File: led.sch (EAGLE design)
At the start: 47 parts, among them U1 TPS92513, U2 TPS92513

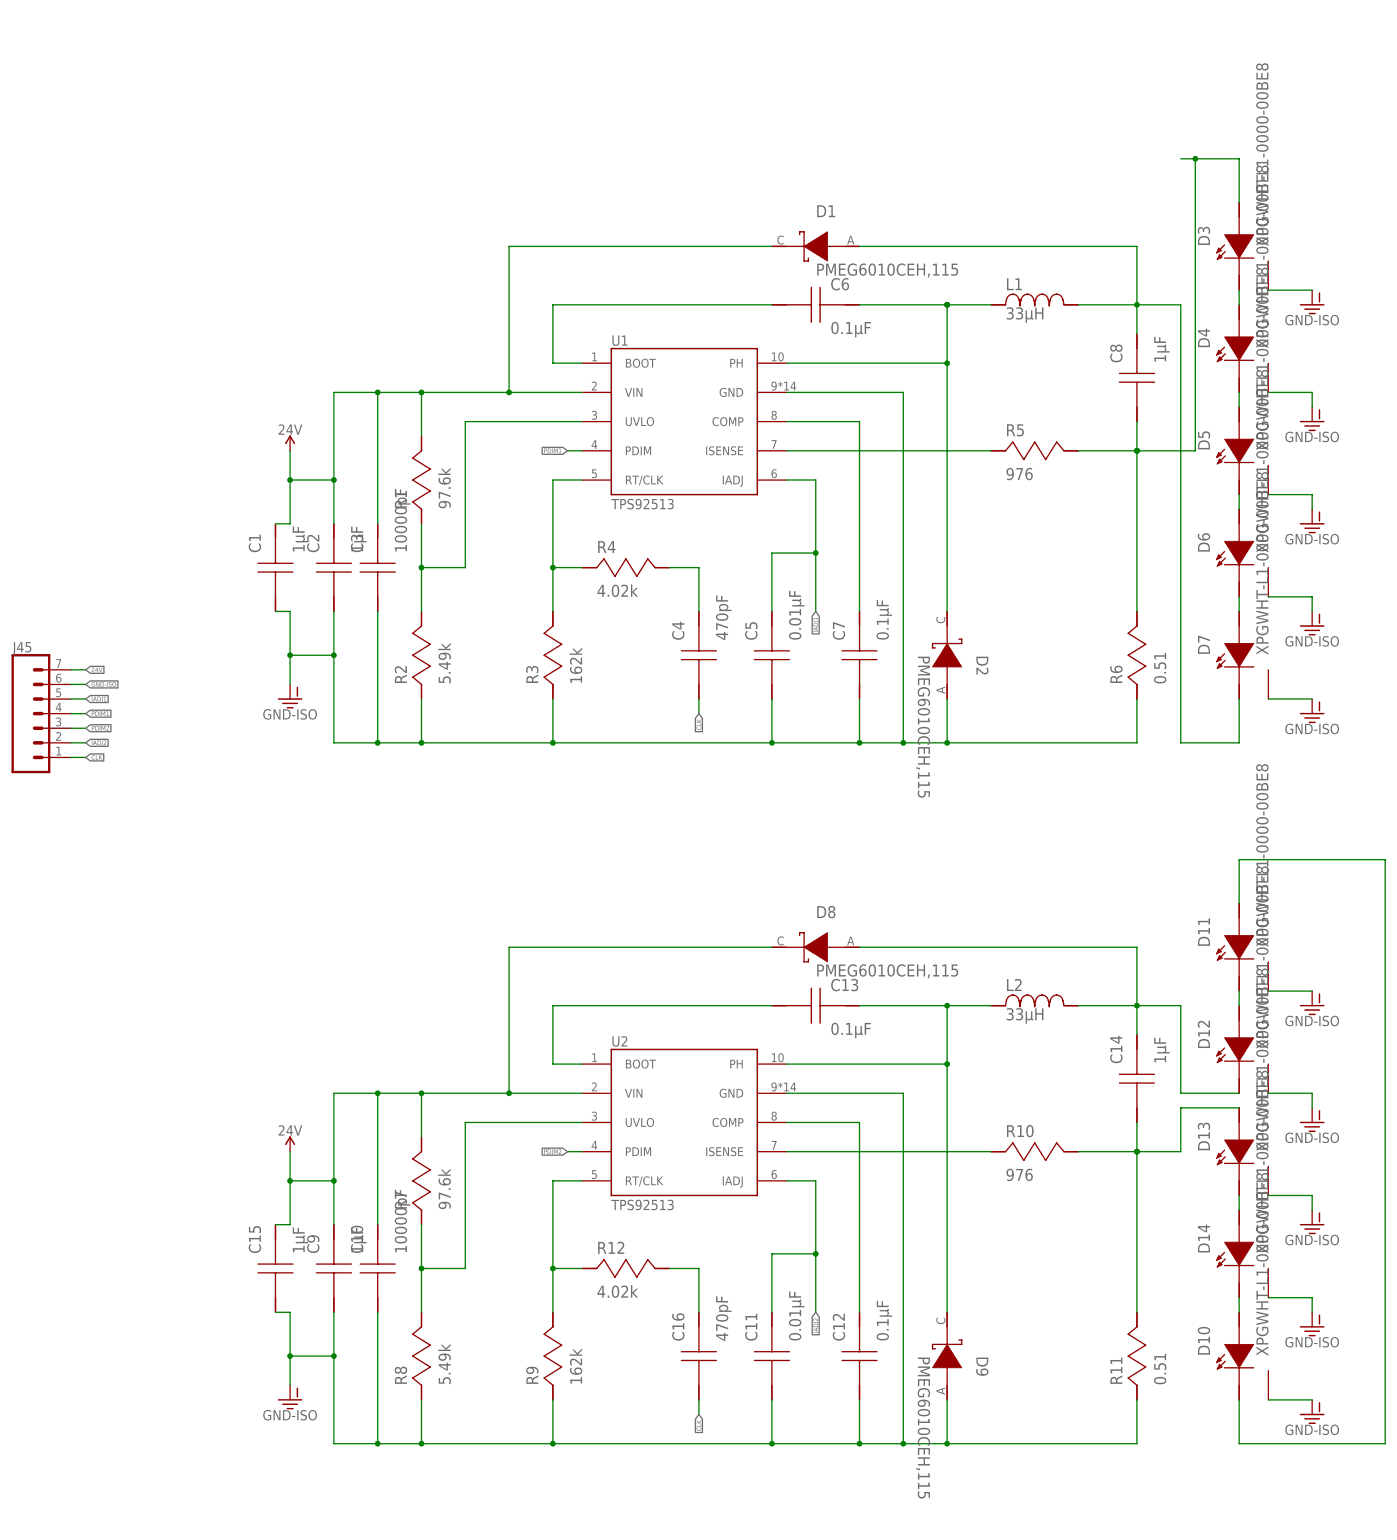
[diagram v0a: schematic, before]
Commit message: save
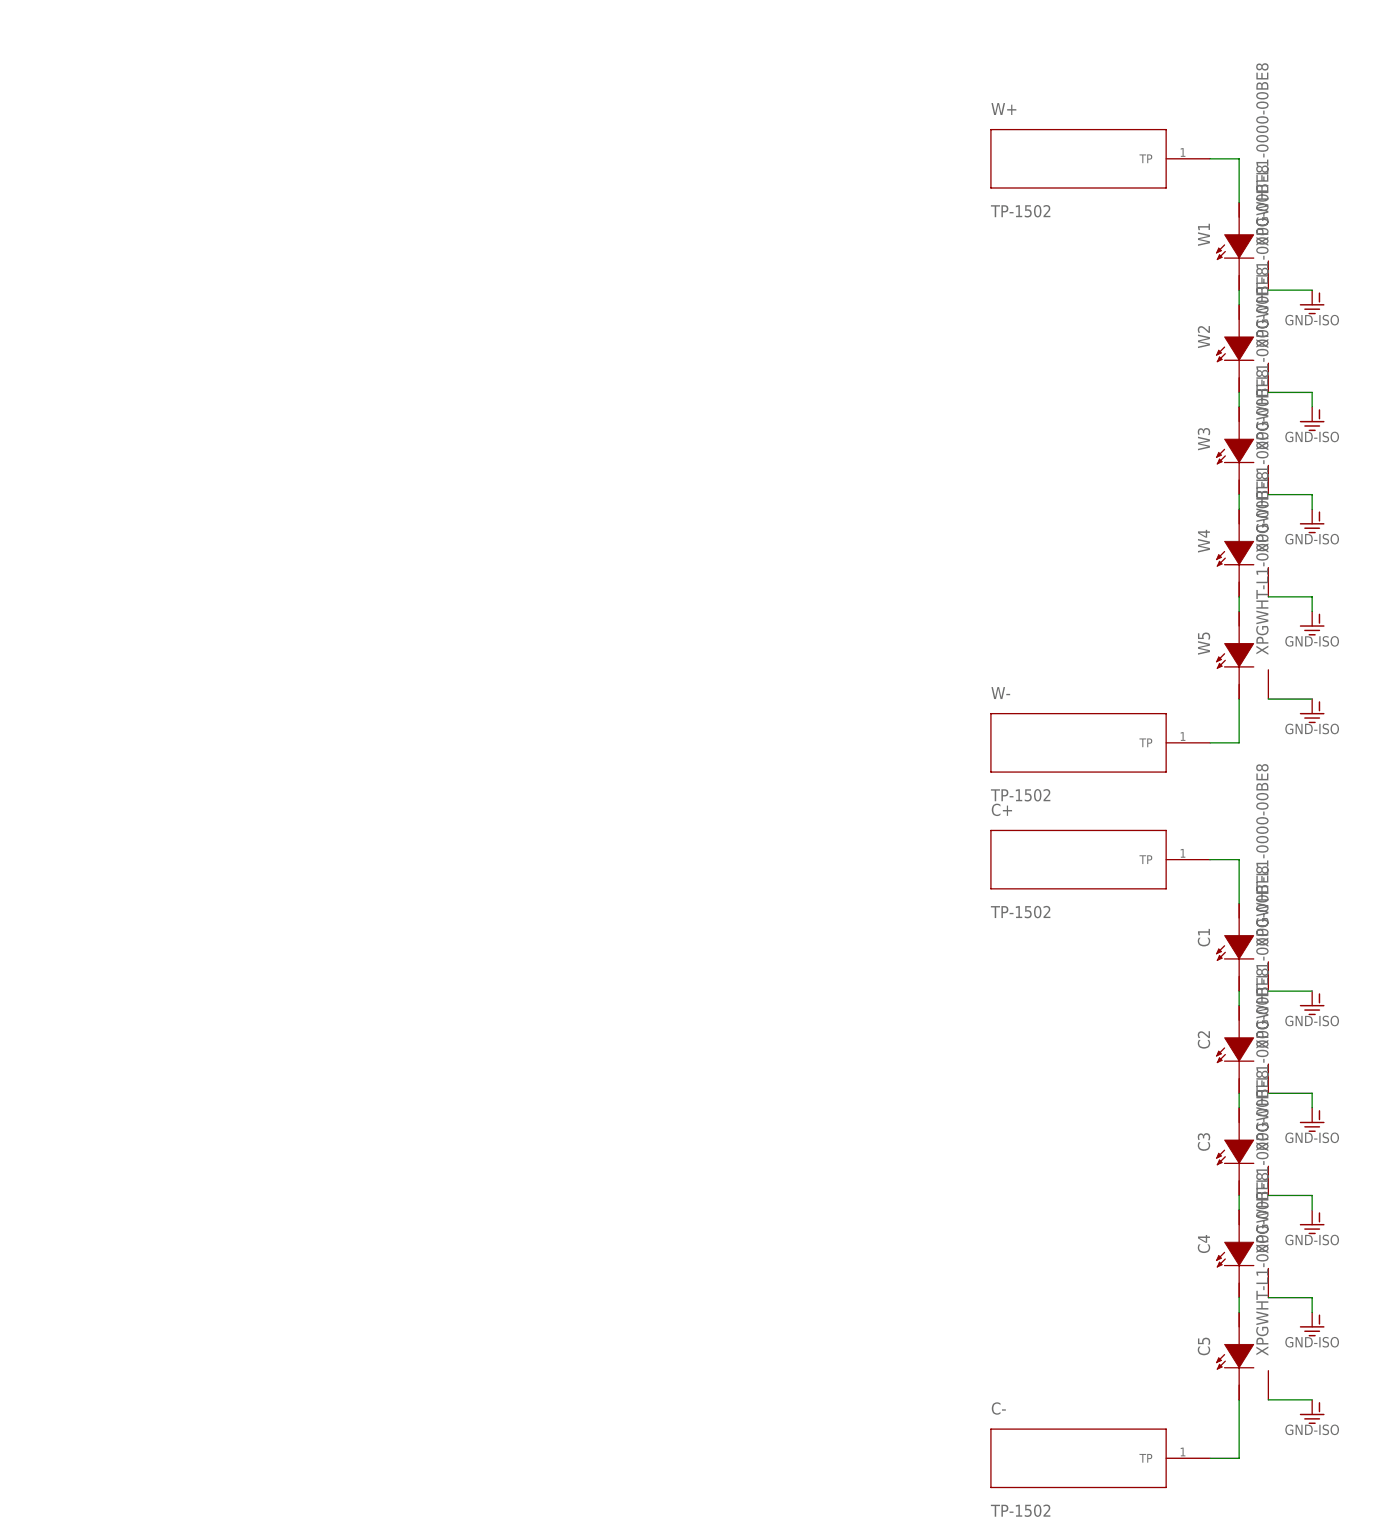
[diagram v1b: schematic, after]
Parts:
- removed C10: 10000pF, derek:GCM155R71H103KA55D
- removed C11: 0.01μF, derek:CC0805KRX7R9BB103
- removed C12, C7: 0.1µF, derek:CC0805KRX7R8BB104
- removed C13, C6: 0.1µF, derek:GRM188R71E104KA01D
- removed C14, C8: 1µF, derek:GMK212B7105KG-T
- removed C15, C9: 1µF, derek:GRM31MR71H105KA88L
- removed C16: 470pF, derek:C0603X471K5RACTU
- removed D1, D2, D8, D9: PMEG6010CEH,115, derek:PMEG6010CEH,115
- removed D10, D11, D12, D13, D14: XPGWHT-L1-0000-00BE8, derek:XPGWHT-L1-0000-00BE8
- removed J45: (no value), derek:CONN_07NO_SILK
- removed L1, L2: 33µH, derek:SRN6045-330M
- removed R1, R7: 97.6k, derek:CRCW040297K6FKED
- removed R10, R5: 976, derek:CRCW0402976RFKED
- removed R11, R6: 0.51, derek:CRM0805-FX-R510ELF
- removed R12, R4: 4.02k, derek:CRCW06034K02FKEA
- removed R2, R8: 5.49k, derek:CRCW04025K49FKED
- removed R3, R9: 162k, derek:CRCW0402162KFKED
- removed U1, U2: TPS92513, derek:TPS92513
- added C+, C-, W+, W-: TP-1502, derek:TP-1502
- C1, C2: value 1µF -> XPGWHT-L1-0000-00BE8; device derek:GRM31MR71H105KA88L -> derek:XPGWHT-L1-0000-00BE8
- C3: value 10000pF -> XPGWHT-L1-0000-00BE8; device derek:GCM155R71H103KA55D -> derek:XPGWHT-L1-0000-00BE8
- C4: value 470pF -> XPGWHT-L1-0000-00BE8; device derek:C0603X471K5RACTU -> derek:XPGWHT-L1-0000-00BE8
- C5: value 0.01μF -> XPGWHT-L1-0000-00BE8; device derek:CC0805KRX7R9BB103 -> derek:XPGWHT-L1-0000-00BE8
- renumbered D3 to W1, D4 to W2, D5 to W3, D6 to W4, D7 to W5
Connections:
- removed net 24V: C1.1, C10.1, C15.1, C2.1, C3.1, C9.1, D1.C, D8.C, J45.7, R1.1, R7.1, U1.VIN, U2.VIN
- removed net CLK: C16.2, C4.2, J45.1
- removed net IADJ1: C5.1, J45.5, U1.IADJ
- removed net IADJ2: C11.1, J45.2, U2.IADJ
- removed net N$10: C6.2, U1.BOOT
- removed net N$11: R5.2, U1.ISENSE
- removed net N$16: C13.1, D9.C, L2.1, U2.PH
- removed net N$17: R12.2, R9.1, U2.RT/CLK
- removed net N$18: C12.1, U2.COMP
- removed net N$19: C13.2, U2.BOOT
- removed net N$20: R10.2, U2.ISENSE
- removed net N$23: C14.1, D12.C, D8.A, L2.2
- removed net N$25: C16.1, R12.1
- removed net N$26: C14.2, D13.A, R10.1, R11.1
- removed net N$27: D10.C, D11.A
- removed net N$34: C4.1, R4.1
- removed net N$5: C6.1, D2.C, L1.1, U1.PH
- removed net N$6: C8.2, R5.1, R6.1, W1.A
- removed net N$7: C8.1, D1.A, L1.2, W5.C
- removed net N$8: R3.1, R4.2, U1.RT/CLK
- removed net N$9: C7.1, U1.COMP
- removed net PDIM1: J45.4, U1.PDIM
- removed net PDIM2: J45.3, U2.PDIM
- new net N$30: W+.TP, W1.A
- new net N$31: W-.TP, W5.C
- new net N$4: C-.TP, C5.C
- net GND-ISO: now also C1.GND, C2.GND, C3.GND, C4.GND, C5.GND; no longer C1.2, C10.2, C11.2, C12.2, C15.2, C2.2, C3.2, C5.2, C7.2, C9.2, D10.GND, D11.GND, D12.GND, D13.GND, D14.GND, D2.A, D9.A, J45.6, R11.2, R2.2, R3.2, R6.2, R8.2, R9.2, U1.GND, U2.GND
- net N$1: now also C2.C, C3.A; no longer R7.2, R8.1, U2.UVLO
- net N$2: now also C1.C, C2.A; no longer D11.C, D12.A
- net N$22: now also C3.C, C4.A; no longer D13.C, D14.A
- net N$24: now also C4.C, C5.A; no longer D10.A, D14.C
- net N$3: now also C+.TP, C1.A; no longer R1.2, R2.1, U1.UVLO

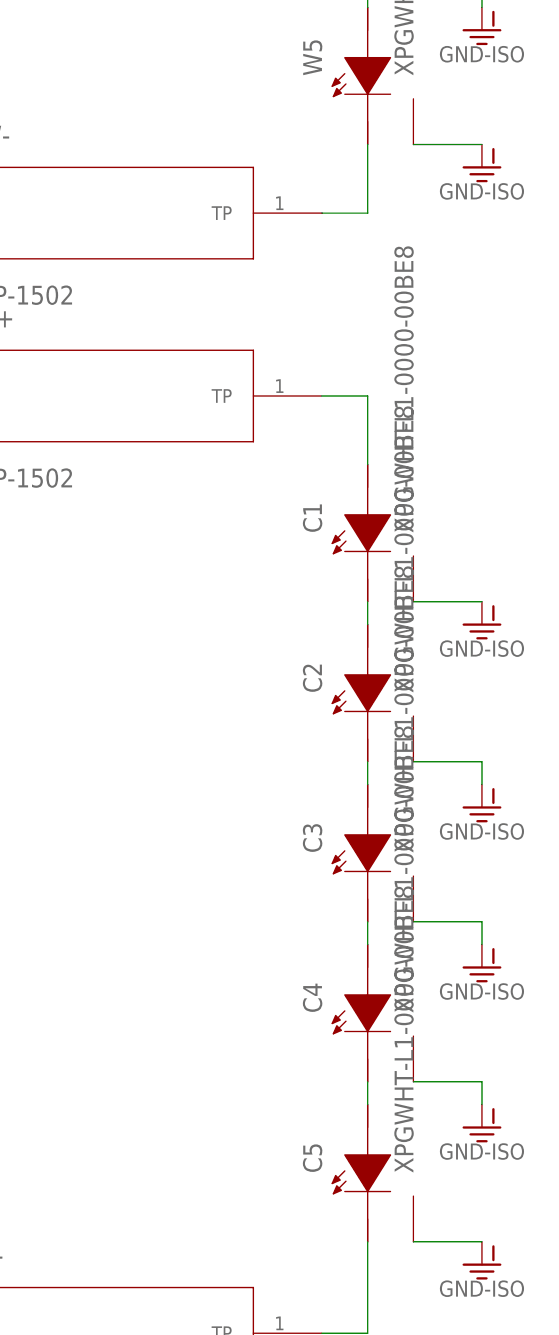
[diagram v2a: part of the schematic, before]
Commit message: use this
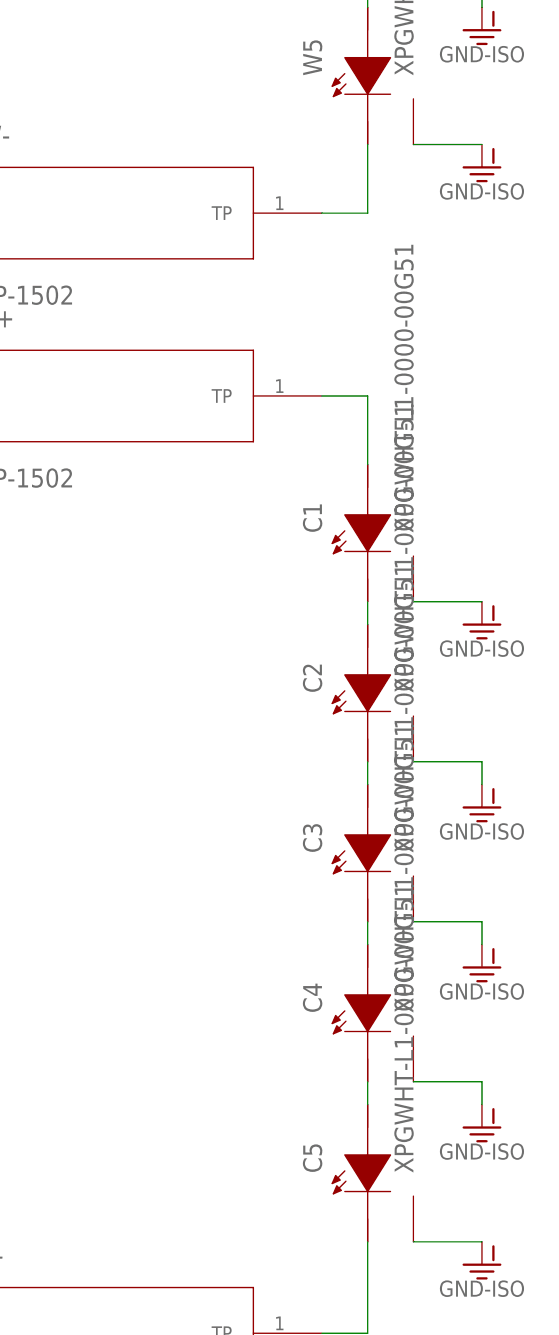
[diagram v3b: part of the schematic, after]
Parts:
- C1, C2, C3, C4, C5: value XPGWHT-L1-0000-00BE8 -> XPGWHT-L1-0000-00G51; device derek:XPGWHT-L1-0000-00BE8 -> derek:XPGWHT-L1-0000-00G51
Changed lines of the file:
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@@
 <grid distance="0.1" unitdist="inch" unit="inch" style="lines" multiple="1" display="no" altdistance="0.01" altunitdist="inch" altunit="inch"/>
 <layers>
-<layer number="1" name="Top" color="4" fill="1" visible="no" active="no"/>
-<layer number="16" name="Bottom" color="1" fill="1" visible="no" active="no"/>
-<layer number="17" name="Pads" color="2" fill="1" visible="no" active="no"/>
-<layer number="18" name="Vias" color="2" fill="1" visible="no" active="no"/>
-<layer number="19" name="Unrouted" color="6" fill="1" visible="no" active="no"/>
-<layer number="20" name="Dimension" color="15" fill="1" visible="no" active="no"/>
-<layer number="21" name="tPlace" color="7" fill="1" visible="no" active="no"/>
-<layer number="22" name="bPlace" color="7" fill="1" visible="no" active="no"/>
-<layer number="23" name="tOrigins" color="15" fill="1" visible="no" active="no"/>
-<layer number="24" name="bOrigins" color="15" fill="1" visible="no" active="no"/>
-<layer number="25" name="tNames" color="7" fill="1" visible="no" active="no"/>
-<layer number="26" name="bNames" color="7" fill="1" visible="no" active="no"/>
-<layer number="27" name="tValues" color="7" fill="1" visible="no" active="no"/>
-<layer number="28" name="bValues" color="7" fill="1" visible="no" active="no"/>
+<layer number="1" name="Top" color="4" fill="1" visible="yes" active="no"/>
+<layer number="16" name="Bottom" color="1" fill="1" visible="yes" active="no"/>
+<layer number="17" name="Pads" color="2" fill="1" visible="yes" active="no"/>
+<layer number="18" name="Vias" color="2" fill="1" visible="yes" active="no"/>
+<layer number="19" name="Unrouted" color="6" fill="1" visible="yes" active="no"/>
+<layer number="20" name="Dimension" color="15" fill="1" visible="yes" active="no"/>
+<layer number="21" name="tPlace" color="7" fill="1" visible="yes" active="no"/>
+<layer number="22" name="bPlace" color="7" fill="1" visible="yes" active="no"/>
+<layer number="23" name="tOrigins" color="15" fill="1" visible="yes" active="no"/>
+<layer number="24" name="bOrigins" color="15" fill="1" visible="yes" active="no"/>
+<layer number="25" name="tNames" color="7" fill="1" visible="yes" active="no"/>
+<layer number="26" name="bNames" color="7" fill="1" visible="yes" active="no"/>
+<layer number="27" name="tValues" color="7" fill="1" visible="yes" active="no"/>
+<layer number="28" name="bValues" color="7" fill="1" visible="yes" active="no"/>
 <layer number="29" name="tStop" color="7" fill="3" visible="no" active="no"/>
 <layer number="30" name="bStop" color="7" fill="6" visible="no" active="no"/>
@@
 <layer number="35" name="tGlue" color="7" fill="4" visible="no" active="no"/>
 <layer number="36" name="bGlue" color="7" fill="5" visible="no" active="no"/>
-<layer number="37" name="tTest" color="7" fill="1" visible="no" active="no"/>
-<layer number="38" name="bTest" color="7" fill="1" visible="no" active="no"/>
+<layer number="37" name="tTest" color="7" fill="1" visible="yes" active="no"/>
+<layer number="38" name="bTest" color="7" fill="1" visible="yes" active="no"/>
 <layer number="39" name="tKeepout" color="4" fill="11" visible="no" active="no"/>
 <layer number="40" name="bKeepout" color="1" fill="11" visible="no" active="no"/>
@@
 <layer number="44" name="Drills" color="7" fill="1" visible="no" active="no"/>
 <layer number="45" name="Holes" color="7" fill="1" visible="no" active="no"/>
-<layer number="46" name="Milling" color="3" fill="1" visible="no" active="no"/>
-<layer number="47" name="Measures" color="7" fill="1" visible="no" active="no"/>
-<layer number="48" name="Document" color="7" fill="1" visible="no" active="no"/>
-<layer number="49" name="Reference" color="7" fill="1" visible="no" active="no"/>
-<layer number="50" name="dxf" color="7" fill="1" visible="no" active="no"/>
-<layer number="51" name="tDocu" color="7" fill="1" visible="no" active="no"/>
-<layer number="52" name="bDocu" color="7" fill="1" visible="no" active="no"/>
-<layer number="53" name="tGND_GNDA" color="7" fill="9" visible="no" active="no"/>
-<layer number="54" name="bGND_GNDA" color="1" fill="9" visible="no" active="no"/>
-<layer number="56" name="wert" color="7" fill="1" visible="no" active="no"/>
-<layer number="57" name="tCAD" color="7" fill="1" visible="no" active="no"/>
-<layer number="59" name="tCarbon" color="7" fill="1" visible="no" active="no"/>
-<layer number="60" name="bCarbon" color="7" fill="1" visible="no" active="no"/>
+<layer number="46" name="Milling" color="3" fill="1" visible="yes" active="no"/>
+<layer number="47" name="Measures" color="7" fill="1" visible="yes" active="no"/>
+<layer number="48" name="Document" color="7" fill="1" visible="yes" active="no"/>
+<layer number="49" name="Reference" color="7" fill="1" visible="yes" active="no"/>
+<layer number="50" name="dxf" color="7" fill="1" visible="yes" active="no"/>
+<layer number="51" name="tDocu" color="7" fill="1" visible="yes" active="no"/>
+<layer number="52" name="bDocu" color="7" fill="1" visible="yes" active="no"/>
+<layer number="53" name="tGND_GNDA" color="7" fill="9" visible="yes" active="no"/>
+<layer number="54" name="bGND_GNDA" color="1" fill="9" visible="yes" active="no"/>
+<layer number="56" name="wert" color="7" fill="1" visible="yes" active="no"/>
+<layer number="57" name="tCAD" color="7" fill="1" visible="yes" active="no"/>
+<layer number="59" name="tCarbon" color="7" fill="1" visible="yes" active="no"/>
+<layer number="60" name="bCarbon" color="7" fill="1" visible="yes" active="no"/>
 <layer number="90" name="Modules" color="5" fill="1" visible="yes" active="yes"/>
 <layer number="91" name="Nets" color="2" fill="1" visible="yes" active="yes"/>
@@
 <part name="GND-ISO49" library="derek" deviceset="GND-ISO" device=""/>
 <part name="GND-ISO50" library="derek" deviceset="GND-ISO" device=""/>
-<part name="C5" library="derek" deviceset="XPGWHT" device="-L1-0000-00BE8" value="XPGWHT-L1-0000-00BE8"/>
-<part name="C1" library="derek" deviceset="XPGWHT" device="-L1-0000-00BE8" value="XPGWHT-L1-0000-00BE8"/>
-<part name="C2" library="derek" deviceset="XPGWHT" device="-L1-0000-00BE8" value="XPGWHT-L1-0000-00BE8"/>
-<part name="C3" library="derek" deviceset="XPGWHT" device="-L1-0000-00BE8" value="XPGWHT-L1-0000-00BE8"/>
-<part name="C4" library="derek" deviceset="XPGWHT" device="-L1-0000-00BE8" value="XPGWHT-L1-0000-00BE8"/>
+<part name="C5" library="derek" deviceset="XPGWHT" device="-L1-0000-00G51" value="XPGWHT-L1-0000-00G51"/>
+<part name="C1" library="derek" deviceset="XPGWHT" device="-L1-0000-00G51" value="XPGWHT-L1-0000-00G51"/>
+<part name="C2" library="derek" deviceset="XPGWHT" device="-L1-0000-00G51" value="XPGWHT-L1-0000-00G51"/>
+<part name="C3" library="derek" deviceset="XPGWHT" device="-L1-0000-00G51" value="XPGWHT-L1-0000-00G51"/>
+<part name="C4" library="derek" deviceset="XPGWHT" device="-L1-0000-00G51" value="XPGWHT-L1-0000-00G51"/>
 <part name="GND-ISO2" library="derek" deviceset="GND-ISO" device=""/>
 <part name="GND-ISO3" library="derek" deviceset="GND-ISO" device=""/>
